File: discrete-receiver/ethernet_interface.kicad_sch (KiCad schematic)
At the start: 22 parts, among them J4 RJ45_Hanrun_HR911105A_Horizon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, J6 SI-52003-F, U11 Ag9905LP, U9 LAN8720A

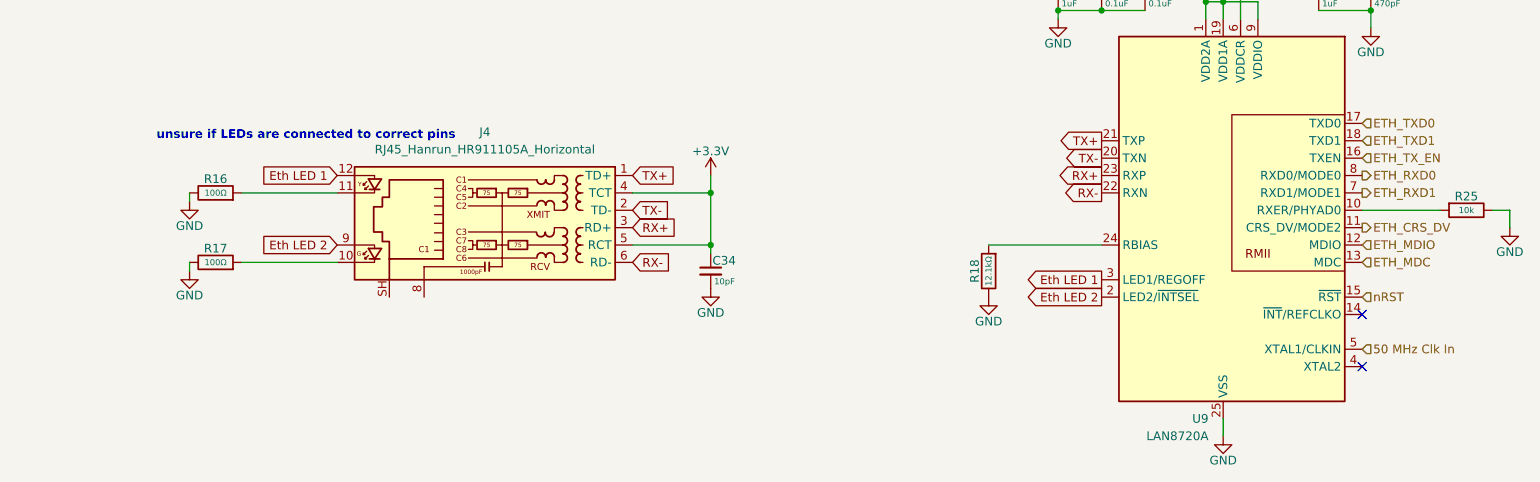
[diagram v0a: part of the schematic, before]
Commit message: Fixed a couple bugs
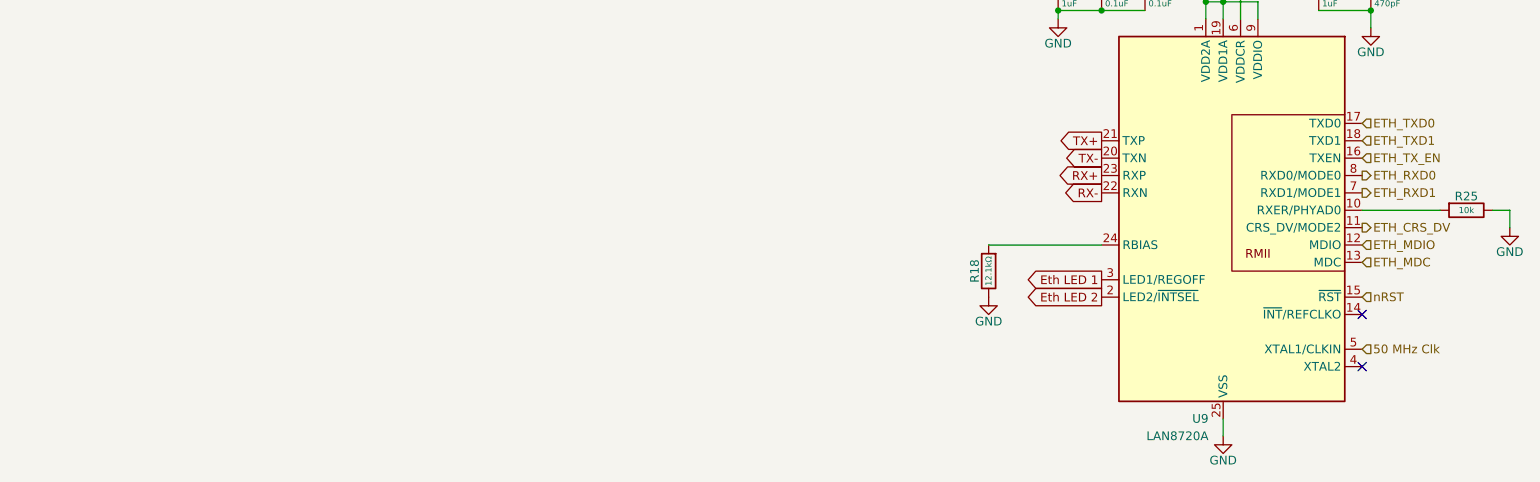
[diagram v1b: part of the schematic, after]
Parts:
- removed C34: 10pF, symbol Device:C_Small
- removed J4: RJ45_Hanrun_HR911105A_Horizontal, Connector_RJ:RJ45_Hanrun_HR911105A_Horizontal, symbol Connector:RJ45_Hanrun_HR911105A_Horizontal
- removed R16, R17: 100Ω, symbol Device:R
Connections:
- net 50 MHz Clk In renamed 50 MHz Clk
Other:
- note removed: "unsure if LEDs are connected to correct pins"
